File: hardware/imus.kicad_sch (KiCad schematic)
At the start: 11 parts, among them U4 ASM330LHHX, U6 IIS2MDCTR

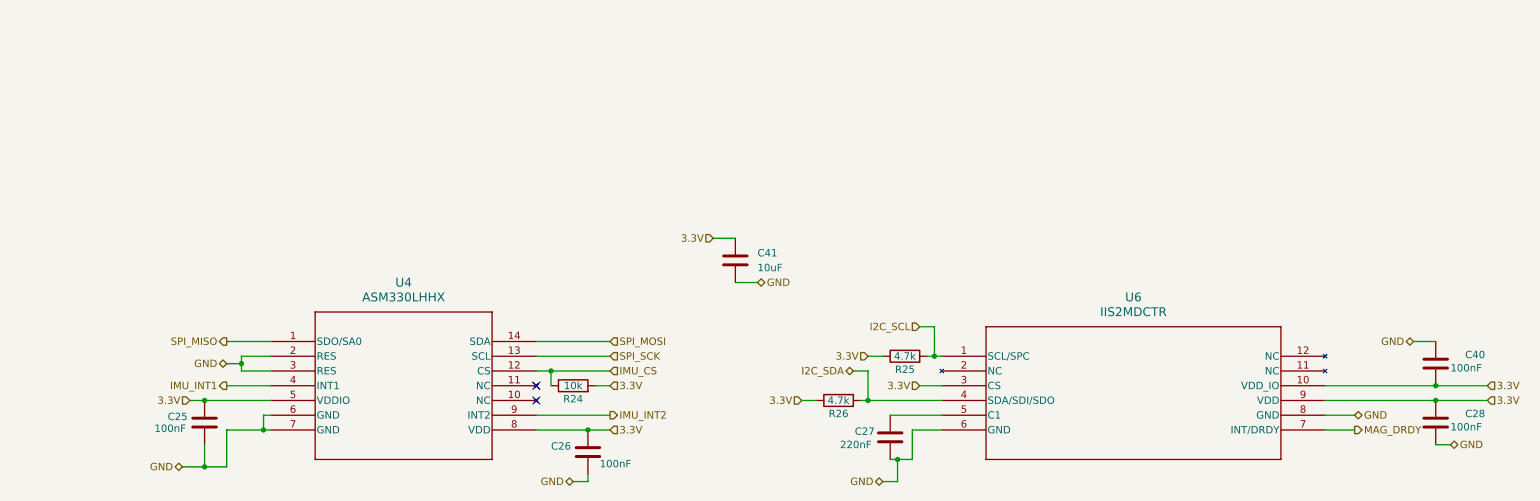
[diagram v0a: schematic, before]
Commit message: Please Final Review
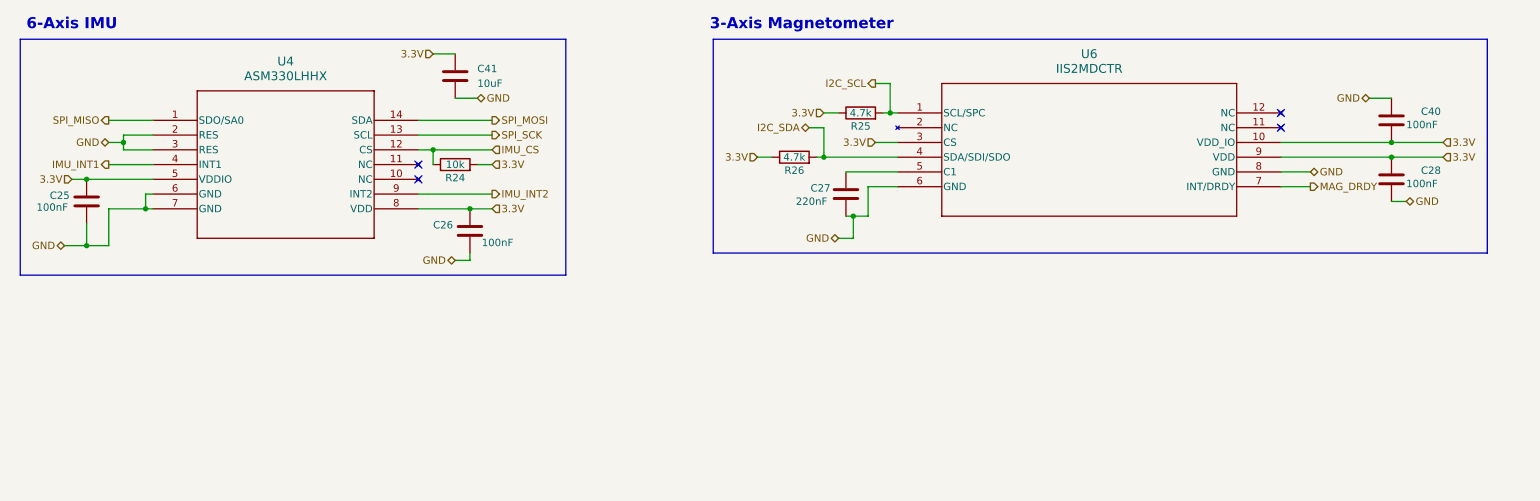
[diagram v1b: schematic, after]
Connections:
- no-connect marks 2 -> 4
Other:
- note added: "3-Axis Magnetometer"
- note added: "6-Axis IMU"
- moved on the sheet: C25, C26, C27, C28, C40, C41, R24, R25, R26, U4, U6
